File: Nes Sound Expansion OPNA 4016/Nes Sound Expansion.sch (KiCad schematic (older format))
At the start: 45 parts, among them J1 NES-SNES Port1, J2 NES-SNES Port2, J3 EXP 1-24, J4 EXP 25-48, J5 EN Switch, J6 AudioJack2_Ground_Switch, J7 EN LED, U1 74LS139, U10 74LS257, U2 74LS132, U6 74LS174, U7 74LS174, U8 74LS257, U9 74LS257, X1 CXO_DIP8

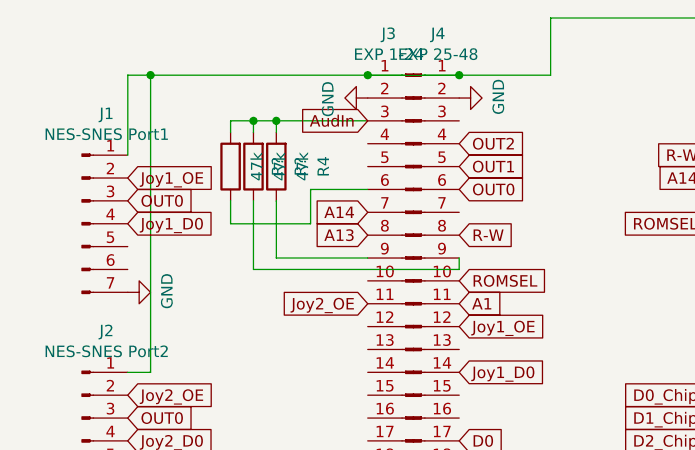
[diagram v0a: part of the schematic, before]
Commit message: minor update
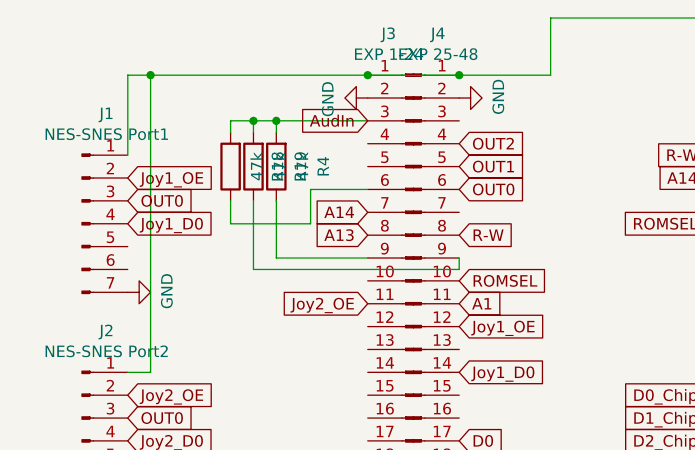
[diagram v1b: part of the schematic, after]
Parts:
- gave numbers to parts that had none: 2
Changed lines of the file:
@@
 A13
 $Comp
-L Device:R R?
+L Device:R R19
 U 1 1 6097469C
 P 1500 1300
-F 0 "R?" V 1293 1300 50  0000 C CNN
+F 0 "R19" V 1293 1300 50  0000 C CNN
 F 1 "47k" V 1384 1300 50  0000 C CNN
 F 2 "Resistor_SMD:R_0805_2012Metric_Pad1.20x1.40mm_HandSolder" V 1430 1300 50  0001 C CNN
@@
 $EndComp
 $Comp
-L Device:R R?
+L Device:R R18
 U 1 1 6097489A
 P 1400 1300
-F 0 "R?" V 1193 1300 50  0000 C CNN
+F 0 "R18" V 1193 1300 50  0000 C CNN
 F 1 "47k" V 1284 1300 50  0000 C CNN
 F 2 "Resistor_SMD:R_0805_2012Metric_Pad1.20x1.40mm_HandSolder" V 1330 1300 50  0001 C CNN
